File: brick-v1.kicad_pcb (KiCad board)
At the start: 2 copper layers, 28 x 41 mm, 15 parts, among them J1 buzzer_toggle_pin, J2 battery_header, U1 Teensy4.1, U2 voltReg

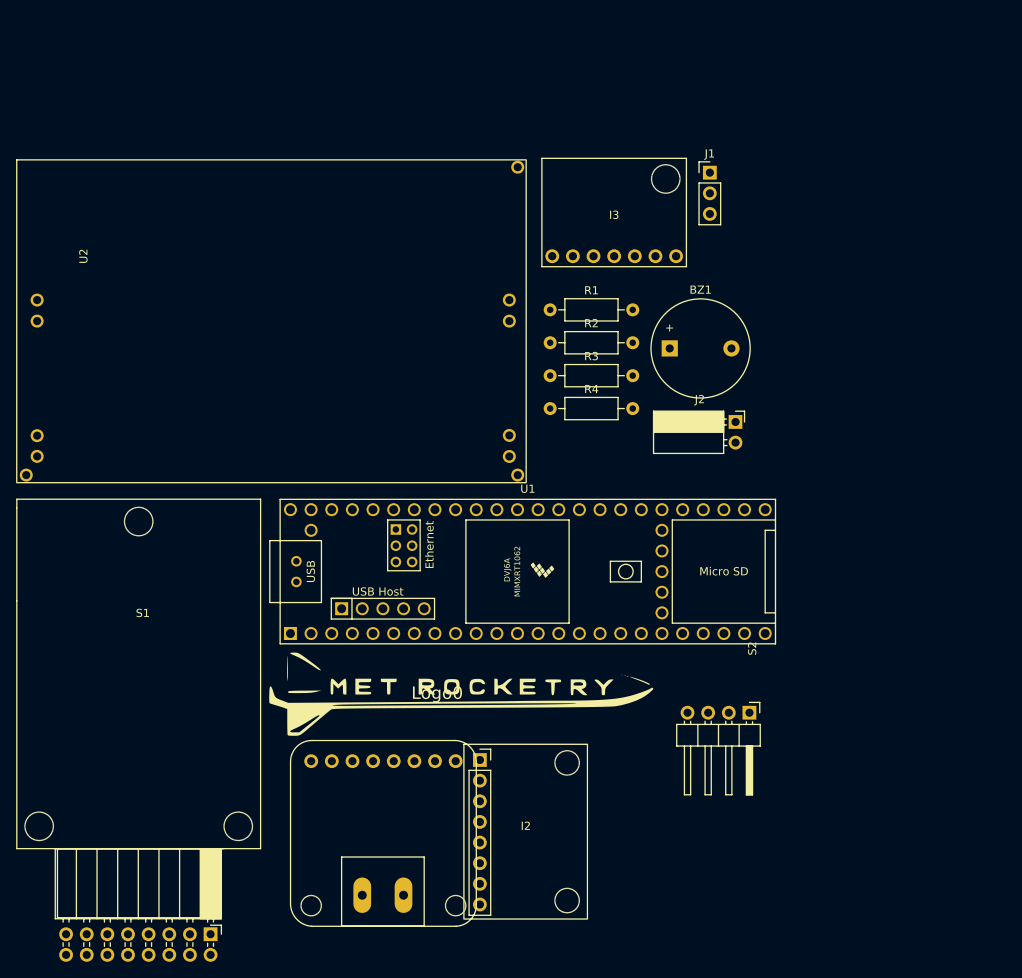
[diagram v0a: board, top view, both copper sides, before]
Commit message: v1.3 update
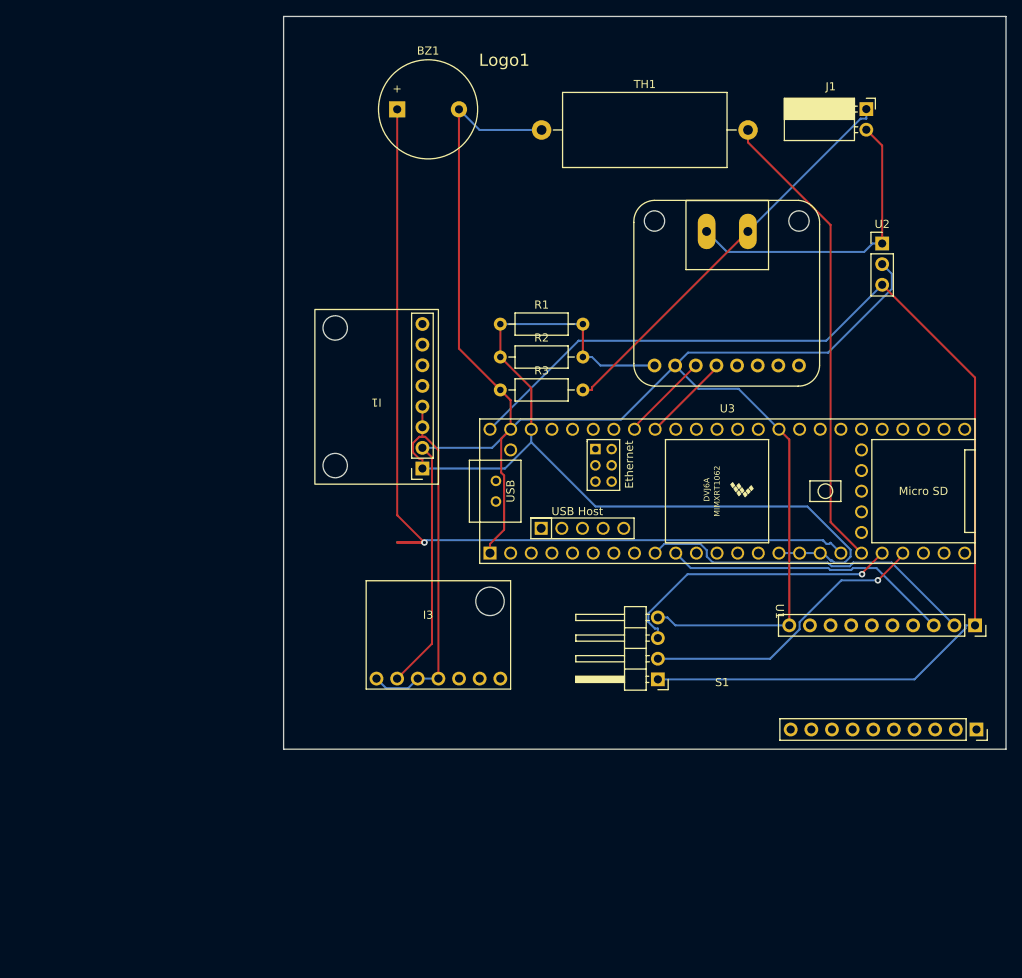
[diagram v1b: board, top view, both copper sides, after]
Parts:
- removed J2: battery_header, Connector_PinSocket_2.54mm:PinSocket_1x02_P2.54mm_Horizontal
- removed Logo0: ~, rrc_logo:RRC_logo
- removed R4: R-Device, Resistor_THT:R_Axial_DIN0207_L6.3mm_D2.5mm_P10.16mm_Horizontal
- removed S2: BN220-GPS, rrc_bn220_gps:BN220
- added Logo1: ~, rrc_logo:tmu, F.Cu at (175.8, 49.8)
- added TH1: Thermistor, Resistor_THT:R_Axial_DIN0922_L20.0mm_D9.0mm_P25.40mm_Horizontal, F.Cu at (179.1, 36.8)
- added U3: Teensy4.1, rrc_teensy:Teensy41, F.Cu at (201.9, 81.3)
- I1: value INA260 -> MPU6050; footprint rrc_INA260:INA260 -> rrc_MPU6050:MPU6050
- I2: value MPU6050 -> INA260; footprint rrc_MPU6050:MPU6050 -> rrc_INA260:INA260
- J1: value buzzer_toggle_pin -> battery_header; footprint Connector_PinHeader_2.54mm:PinHeader_1x03_P2.54mm_Vertical -> Connector_PinSocket_2.54mm:PinSocket_1x02_P2.54mm_Horizontal
- S1: value RFD900+-RF_Module -> BN220-GPS; footprint rrc_rfd900+:RFD900+ -> rrc_bn220_gps:BN220
- U1: value Teensy4.1 -> XB3-24Z8CM-J; footprint rrc_teensy:Teensy41 -> RRC_footprint:xbee_s2c
- U2: value voltReg -> L7805; footprint rrc_voltReg:voltReg2 -> Connector_PinHeader_2.54mm:PinHeader_1x03_P2.54mm_Vertical
- moved U2 107.0 mm to (221.0, 50.8)
- moved S1 71.0 mm to (175.9, 89.6)
- moved I2 70.4 mm to (201.9, 57.1)
- moved I3 56.3 mm to (166.4, 108.2)
- moved I1 53.3 mm to (158.8, 69.8)
- moved BZ1 44.6 mm to (161.3, 34.3)
- moved U1 30.9 mm to (207.9, 96.1), turned to -90 degrees
- moved J1 20.8 mm to (219.0, 34.3)
- moved R1 6.38 mm to (174.0, 60.7)
- moved R2 6.38 mm to (174.0, 64.8)
- moved R3 6.38 mm to (174.0, 68.8)
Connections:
- I1 pad 1: Net-(I1-VIN+) -> SCL2
- I1 pad 2: /V+ -> GND
- I1 pad 3: T_VCC -> SCL2
- I1 pad 4: GND -> SCL2
- I1 pad 5: SCL -> unconnected-(I1-XDA-Pad5)
- I1 pad 6: SDA -> unconnected-(I1-XCL-Pad6)
- I2 pad 1: T_VCC -> /V+
- I2 pad 2: GND -> /V-
- I2 pad 3: SCL1 -> SCL2
- I2 pad 4: SDA1 -> GND
- I2 pad 5: unconnected-(I2-XDA-Pad5) -> SCL
- I2 pad 6: unconnected-(I2-XCL-Pad6) -> SDA
- I3 pad 1: T_VCC -> SCL2
- I3 pad 4: SDA2 -> SCL2
- J1 pad 1: GND -> /V-
- J1 pad 2: Net-(J1-Pin_2) -> /V+
- R1 pad 1: SDA1 -> SCL2
- R1 pad 2: T_VCC -> SCL2
- R2 pad 1: SCL1 -> SCL2
- R2 pad 2: T_VCC -> SCL2
- R3 pad 1: SCL2 -> GND
- R3 pad 2: T_VCC -> /V-
- S1 pad 1: GND -> VCC
- S1 pad 2: GND -> TX7
- S1 pad 3: unconnected-(S1-SICTS-Pad3) -> RX7
- S1 pad 4: VCC -> GND
- U1 pad 10: unconnected-(U1-10_CS_MQSR-Pad10) -> GND
- U1 pad 2: unconnected-(U1-2_OUT2-Pad2) -> VCC
- U1 pad 22: unconnected-(U1-22_A8_CTX1-Pad22) -> (no net)
- U1 pad 30: unconnected-(U1-30_CRX3-Pad30) -> TX2
- U1 pad 31: unconnected-(U1-31_CTX3-Pad31) -> RX2
- U1 pad 33: unconnected-(U1-33_MCLK2-Pad33) -> (no net)
- U1 pad 66: unconnected-(U1-D--Pad66) -> (no net)
- U1 pad 7: RX2 -> unconnected-(U1-RSSI_PWM/DIO10-Pad7)
- U1 pad 8: TX2 -> unconnected-(U1-PWM1/DIO11-Pad8)
- U2 pad 2: /V- -> GND
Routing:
- net GND: track 0.00 -> 227.2 mm
- net SCL2: track 0.00 -> 157.9 mm
- net VCC: track 0.00 -> 144.3 mm
- net Net-(BZ1--): track 0.00 -> 120.3 mm, vias 0 -> 1
- net Net-(U3-27_A13_SCK1): track 0.00 -> 57.9 mm
- net /V-: track 0.00 -> 50.1 mm
- net RX2: track 0.00 -> 42.5 mm
- net /V+: track 0.00 -> 37.9 mm
- net TX7: track 0.00 -> 36.2 mm, vias 0 -> 1
- net RX7: track 0.00 -> 35.7 mm, vias 0 -> 1
- net TX2: track 0.00 -> 35.6 mm
- net SDA: track 0.00 -> 11.0 mm
- net SCL: track 0.00 -> 11.0 mm
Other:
- board size 28 x 41 mm -> 88.9 x 90.2 mm
